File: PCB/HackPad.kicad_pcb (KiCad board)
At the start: 2 copper layers, 63.8 x 83.5 mm, 30 parts, among them J1 Conn_01x04, SW1 SW_Push, SW10 SW_Push, SW2 SW_Push, SW3 SW_Push, SW4 SW_Push, SW5 RotaryEncoder_Switch, SW6 SW_Push, SW7 SW_Push, SW8 SW_Push, SW9 SW_Push, U1 XIAO-RP2040-DIP

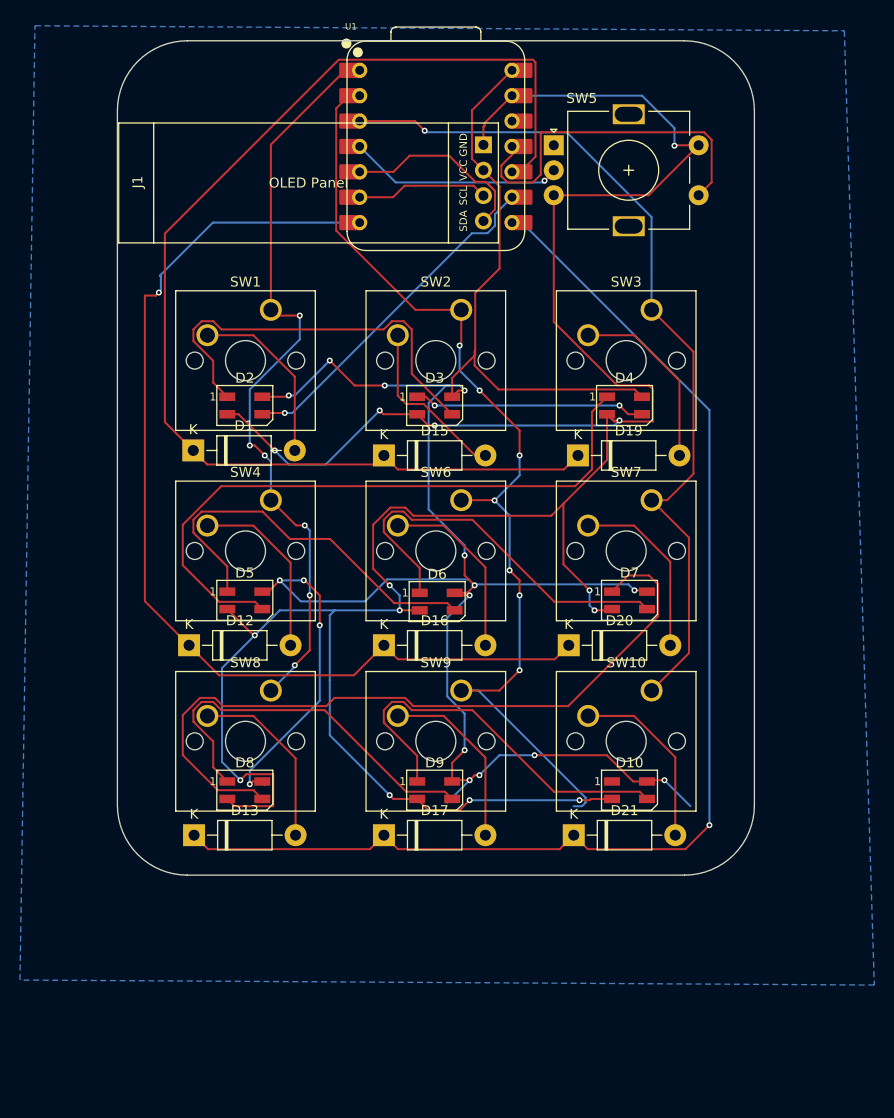
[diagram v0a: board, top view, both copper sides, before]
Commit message: Update HackPad.kicad_pcb
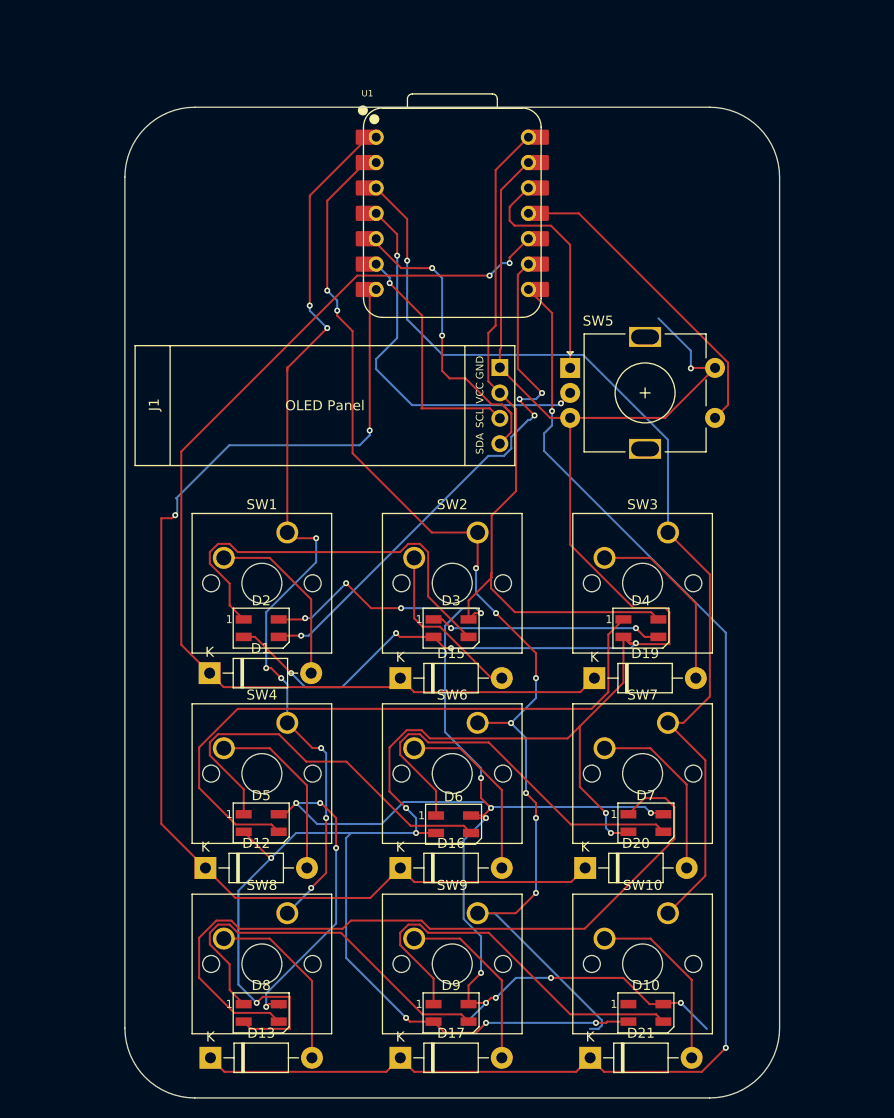
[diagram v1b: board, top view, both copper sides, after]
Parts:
- moved SW4 22.3 mm to (173.2, 86.3)
- moved SW6 22.3 mm to (192.3, 86.3)
- moved SW5 22.3 mm to (201.6, 50.7)
- moved SW7 22.3 mm to (211.3, 86.3)
- moved D10 22.3 mm to (209.1, 115.3)
- moved D12 22.3 mm to (165.1, 100.8)
- moved D13 22.3 mm to (165.6, 119.8)
- moved D15 22.3 mm to (184.6, 81.8)
- moved D16 22.3 mm to (184.6, 100.8)
- moved D17 22.3 mm to (184.6, 119.8)
- moved D2 22.3 mm to (170.6, 76.8)
- moved D20 22.3 mm to (203.1, 100.8)
- moved D21 22.3 mm to (203.6, 119.8)
- moved D3 22.3 mm to (189.6, 76.8)
- moved D4 22.3 mm to (208.6, 76.8)
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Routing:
- net +3V3: track 0.00 -> 23.4 mm
- net Yay: track 34.4 -> 54.3 mm, vias 1 -> 4
- net Net-(U1-GPIO27/ADC1/A1): track 100.4 -> 118.1 mm, vias 7 -> 9
- net Net-(U1-GPIO29/ADC3/A3): track 21.5 -> 38.8 mm, vias 1 -> 2
- net Net-(U1-GPIO26/ADC0/A0): track 76.1 -> 93.1 mm, vias 6 -> 8
- net Net-(D12-K): track 104.0 -> 120.1 mm, vias 1 -> 2
- net Net-(D13-K): track 124.6 -> 140.2 mm, vias 1 -> 2
- net +5V: track 229.2 -> 244.8 mm
- net Net-(U1-GPIO28/ADC2/A2): track 88.1 -> 100.4 mm
- net GND: track 273.6 -> 285.3 mm
- net Net-(D1-K): track 119.5 -> 107.9 mm, vias 0 -> 2
- net SCL: track 13.3 -> 24.6 mm, vias 0 -> 1
- net SDA: track 20.1 -> 30.9 mm, vias 0 -> 2
- net Net-(U1-GPIO3/MOSI): track 36.0 -> 32.2 mm
- removed copper zone on B.Cu, net GND
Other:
- board size 63.8 x 83.5 mm -> 65.5 x 99.2 mm
